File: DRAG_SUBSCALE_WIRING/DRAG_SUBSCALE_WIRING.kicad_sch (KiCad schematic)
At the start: 7 parts, among them J1 Screw_Terminal_01x02, SW1 SW_DPST_x2, U1 Teensy4.1

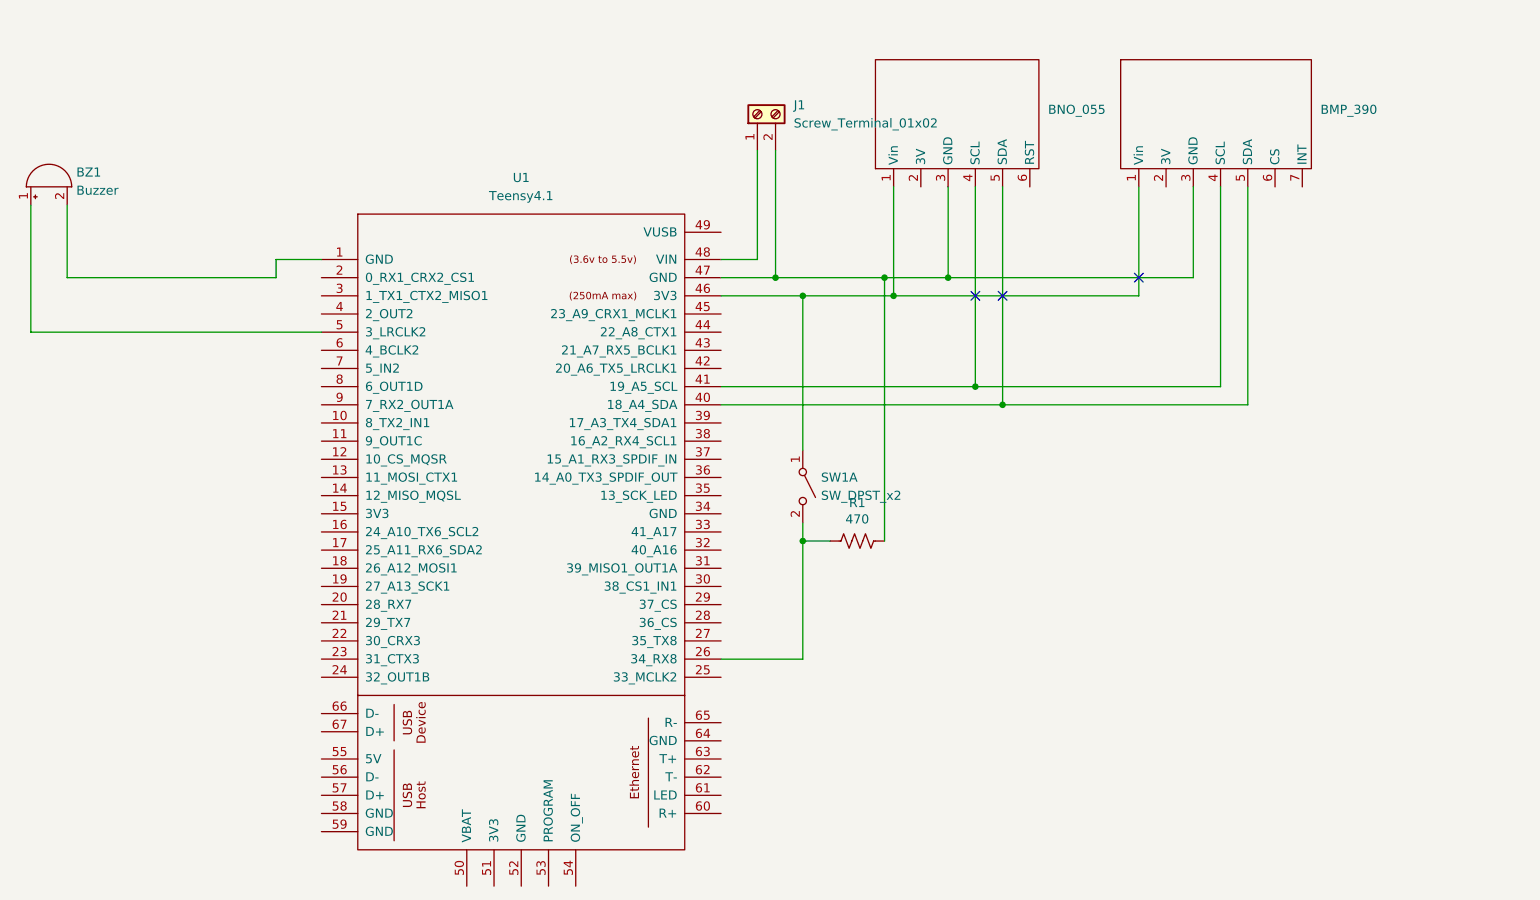
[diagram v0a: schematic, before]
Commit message: worked on pcb and adding 3d models
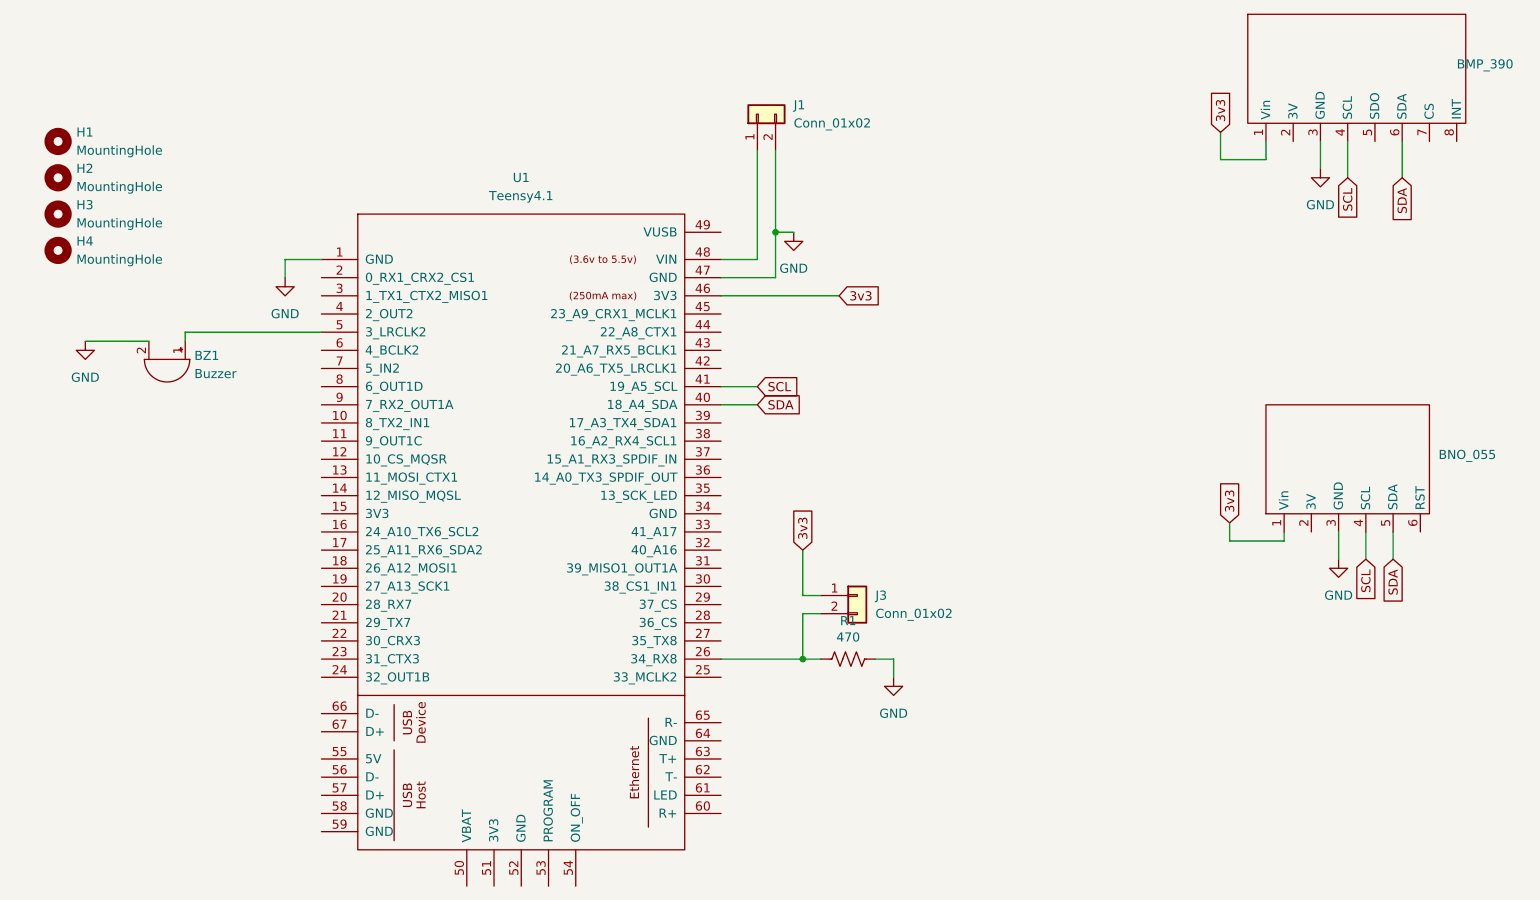
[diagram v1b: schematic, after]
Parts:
- removed J1: Screw_Terminal_01x02, symbol Connector:Screw_Terminal_01x02
- removed SW1: SW_DPST_x2, symbol Switch:SW_DPST_x2
- added H1, H2, H3, H4: MountingHole, MountingHole:MountingHole_3.2mm_M3_DIN965, symbol Mechanical:MountingHole
- added J1, J3: Conn_01x02, Connector_JST:JST_XA_B02B-XASK-1_1x02_P2.50mm_Vertical, symbol Connector_Generic:Conn_01x02
- BMP_390: footprint (none) -> Breakouts:BMP390
- BNO_055: footprint (none) -> Breakouts:BNO055Ada
- BZ1: footprint (none) -> Buzzer_Beeper:Buzzer_TDK_PS1240P02BT_D12.2mm_H6.5mm
- R1: footprint (none) -> Resistor_THT:R_Axial_DIN0411_L9.9mm_D3.6mm_P15.24mm_Horizontal
- U1: footprint (none) -> Breakouts:Teensy41
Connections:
- net 3v3: now reaches BMP_390.1 (Vin), BNO_055.1 (Vin), U1.46 (3V3)
- net 3v3: now also J3.1 (Pin_1)
- net GND: now reaches BMP_390.3 (GND), BNO_055.3 (GND), R1.2, U1.47 (GND)
- net GND: now also BZ1.2 (-), U1.1 (GND), J1.2 (Pin_2)
- net SCL: now reaches BMP_390.4 (SCL), BNO_055.4 (SCL), U1.41 (19_A5_SCL)
- net SDA: now reaches BNO_055.5 (SDA), U1.40 (18_A4_SDA)
- net SDA: now also BMP_390.6 (SDA); no longer BMP_390.5 (SDA)
- net at R1.1, U1.26 (34_RX8): now also J3.2 (Pin_2)
- net at U1.48 (VIN): now also J1.1 (Pin_1)
- no-connect marks 3 -> 0
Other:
- moved on the sheet: BNO_055, BZ1, R1
